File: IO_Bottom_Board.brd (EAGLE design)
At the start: 112.7 x 50.8 mm, 16 parts, among them IC1 L293D, IC2 L293D, T1 BPX81, U1 LM324PW

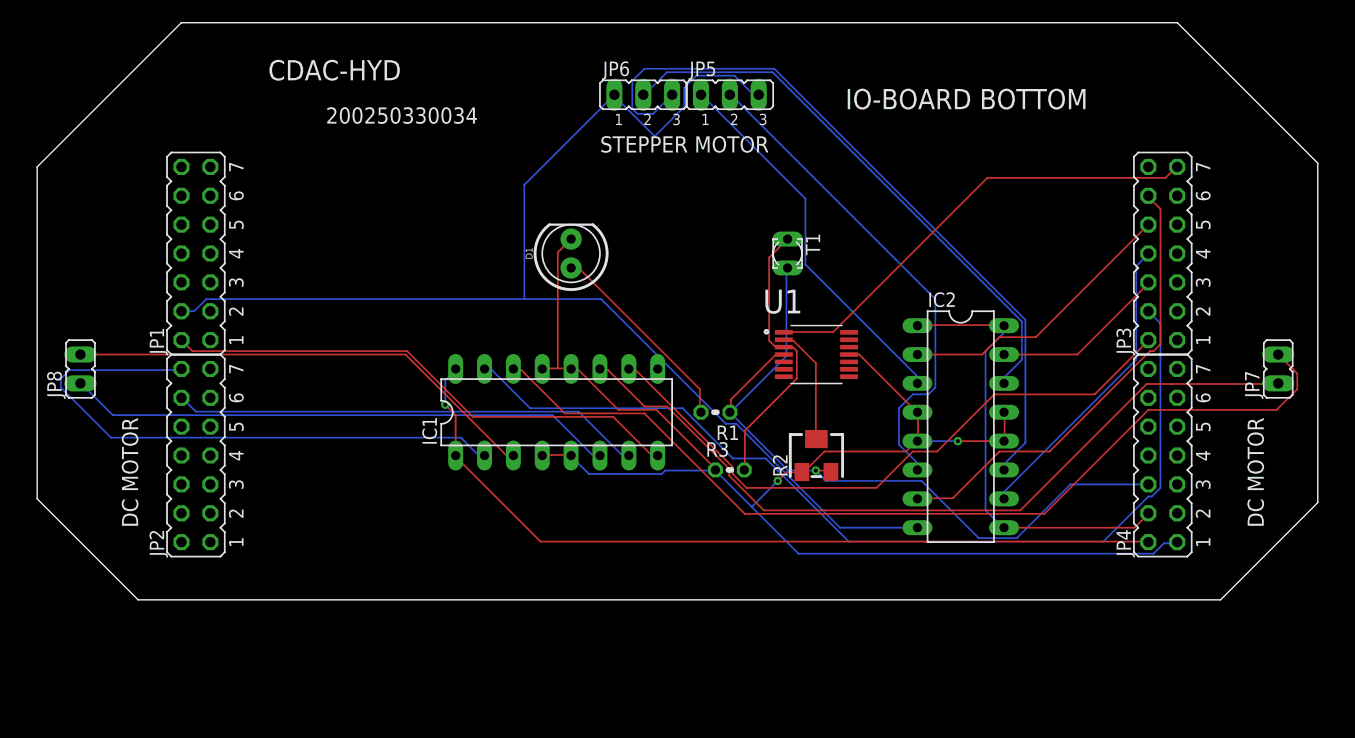
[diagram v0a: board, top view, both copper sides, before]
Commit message: Add files via upload
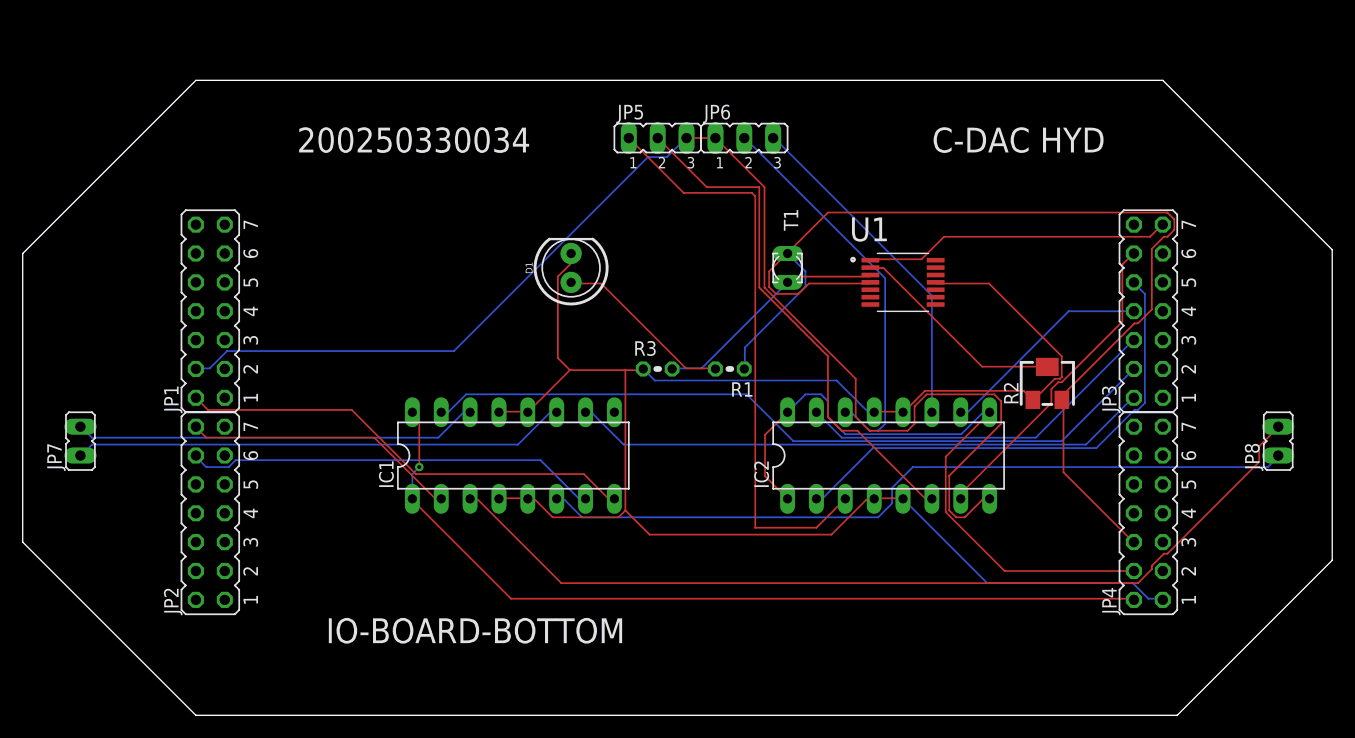
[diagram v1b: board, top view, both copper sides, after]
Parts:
- moved JP7 105.6 mm to (8.89, 38.1)
- moved JP8 105.6 mm to (114.3, 38.1)
- moved R2 21.3 mm to (94.0, 43.2)
- moved R3 10.9 mm to (59.7, 44.5)
- moved U1 9.92 mm to (81.3, 52.1)
- moved JP6 9.67 mm to (67.3, 64.8)
- moved JP5 7.41 mm to (59.7, 64.8)
- moved IC2 6.84 mm to (80.0, 36.8), turned to 0 degrees
- moved IC1 5.39 mm to (47.0, 36.8)
- moved JP1 5.24 mm to (20.3, 49.5)
- moved JP2 5.24 mm to (20.3, 31.8)
- moved JP3 5.24 mm to (102.9, 49.5)
- moved JP4 5.24 mm to (102.9, 31.8)
- moved R1 4.02 mm to (66.0, 44.5)
- moved D1 1.27 mm to (52.1, 53.3)
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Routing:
- net N$4: track 82.6 -> 35.6 mm
- net N$1: track 41.8 -> 80.9 mm
- net N$17: track 65.0 -> 30.0 mm
- net N$22: track 67.1 -> 97.7 mm, vias 1 -> 0
- net GND: track 129.2 -> 159.3 mm, vias 2 -> 0
- net N$5: track 51.5 -> 24.2 mm
- net N$3: track 69.9 -> 43.5 mm
- net N$14: track 40.1 -> 59.9 mm
- net N$2: track 48.3 -> 67.3 mm
- net N$12: track 25.1 -> 43.4 mm
- net N$16: track 33.3 -> 51.4 mm
- net N$8: track 83.7 -> 65.9 mm
- net N$10: track 15.4 -> 32.4 mm
- net N$19: track 49.3 -> 34.8 mm
- net N$21: track 40.6 -> 27.0 mm
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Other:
- board size 112.7 x 50.8 mm -> 115.2 x 55.9 mm
- board text added: "C-DAC HYD"
- board text added: "IO-BOARD-BOTTOM"
- board text removed: "CDAC-HYD"
- board text removed: "DC MOTOR"
- board text removed: "IO-BOARD BOTTOM"
- board text removed: "STEPPER MOTOR"
